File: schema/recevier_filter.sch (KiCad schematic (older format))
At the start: 14 parts, among them U7 LM358, U8 LM393

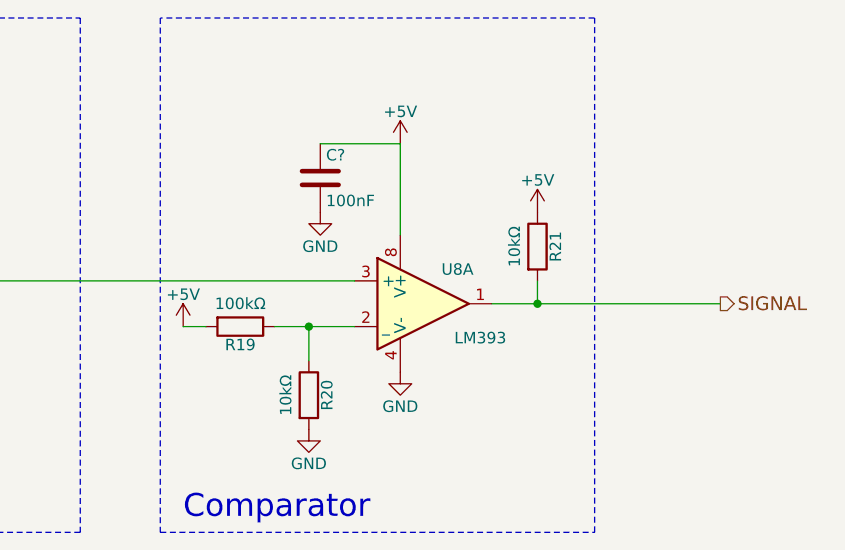
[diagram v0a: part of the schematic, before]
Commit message: Reception: schmidt trigger
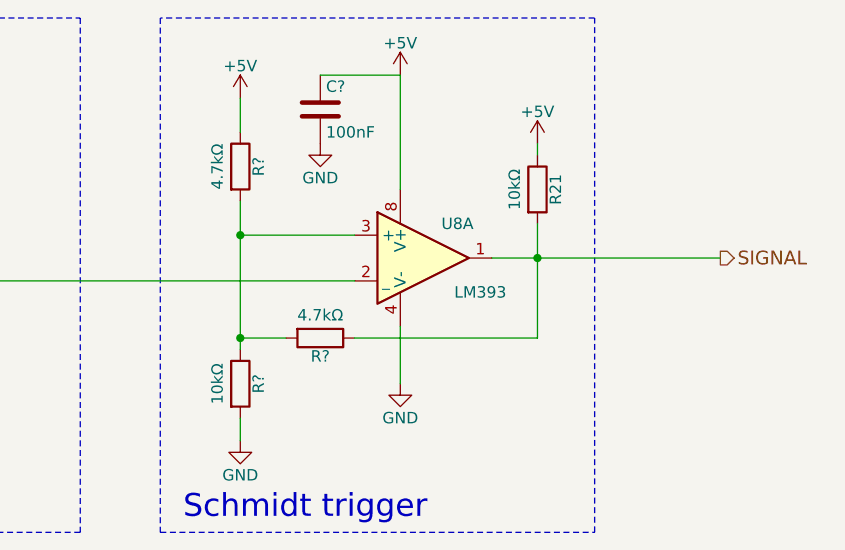
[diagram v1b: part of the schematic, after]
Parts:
- removed R19: 100kΩ, symbol R
- removed R20: 10kΩ, symbol R
- added R? (x2): 4.7kΩ, symbol R
- added R?: 10kΩ, symbol R
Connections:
- net +5V: now also R?.1
- net GND: now also R?.2
- net SIGNAL: now also R?.1
- net at R18.1, U?.1: now also U8.2 (_); no longer U8.3 (+)
- new net: R?.1, R?.2, R?.2, U8.3 (+)
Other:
- note added: "Schmidt trigger"
- note removed: "Comparator"
- moved on the sheet: C?, R21, U8A
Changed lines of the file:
@@
 Comment4 ""
 $EndDescr
-Text HLabel 9700 3650 2    60   Output ~ 0
+Text HLabel 9700 3450 2    60   Output ~ 0
 SIGNAL
 $Comp
@@
 L LM393 U8
 U 1 1 5924C9D9
-P 8400 3650
-F 0 "U8" H 8550 3800 50  0000 C CNN
-F 1 "LM393" H 8650 3500 50  0000 C CNN
-F 2 "" H 8400 3650 50  0000 C CNN
-F 3 "" H 8400 3650 50  0000 C CNN
-	1    8400 3650
-	1    0    0    -1
-$EndComp
-$Comp
-L R R19
-U 1 1 5924CC18
-P 7600 3750
-F 0 "R19" V 7680 3750 50  0000 C CNN
-F 1 "100kΩ" V 7500 3750 50  0000 C CNN
-F 2 "" V 7530 3750 50  0000 C CNN
-F 3 "" H 7600 3750 50  0000 C CNN
-	1    7600 3750
-	0    1    1    0
-$EndComp
-$Comp
-L R R20
-U 1 1 5924CC6A
-P 7900 4050
-F 0 "R20" V 7980 4050 50  0000 C CNN
-F 1 "10kΩ" V 7800 4050 50  0000 C CNN
-F 2 "" V 7830 4050 50  0000 C CNN
-F 3 "" H 7900 4050 50  0000 C CNN
-	1    7900 4050
+P 8400 3450
+F 0 "U8" H 8550 3600 50  0000 C CNN
+F 1 "LM393" H 8650 3300 50  0000 C CNN
+F 2 "" H 8400 3450 50  0000 C CNN
+F 3 "" H 8400 3450 50  0000 C CNN
+	1    8400 3450
 	1    0    0    -1
 $EndComp
@@
 L GND #PWR23
 U 1 1 5924CCA3
-P 7900 4200
-F 0 "#PWR23" H 7900 3950 50  0001 C CNN
-F 1 "GND" H 7900 4050 50  0000 C CNN
-F 2 "" H 7900 4200 50  0000 C CNN
-F 3 "" H 7900 4200 50  0000 C CNN
-	1    7900 4200
+P 7600 4250
+F 0 "#PWR23" H 7600 4000 50  0001 C CNN
+F 1 "GND" H 7600 4100 50  0000 C CNN
+F 2 "" H 7600 4250 50  0000 C CNN
+F 3 "" H 7600 4250 50  0000 C CNN
+	1    7600 4250
 	1    0    0    -1
 $EndComp
@@
 L GND #PWR25
 U 1 1 5924CE19
-P 8300 3950
-F 0 "#PWR25" H 8300 3700 50  0001 C CNN
-F 1 "GND" H 8300 3800 50  0000 C CNN
-F 2 "" H 8300 3950 50  0000 C CNN
-F 3 "" H 8300 3950 50  0000 C CNN
-	1    8300 3950
+P 8300 4000
+F 0 "#PWR25" H 8300 3750 50  0001 C CNN
+F 1 "GND" H 8300 3850 50  0000 C CNN
+F 2 "" H 8300 4000 50  0000 C CNN
+F 3 "" H 8300 4000 50  0000 C CNN
+	1    8300 4000
 	1    0    0    -1
 $EndComp
@@
 L +5V #PWR24
 U 1 1 5924CE97
-P 8300 2950
-F 0 "#PWR24" H 8300 2800 50  0001 C CNN
-F 1 "+5V" H 8300 3090 50  0000 C CNN
-F 2 "" H 8300 2950 50  0000 C CNN
-F 3 "" H 8300 2950 50  0000 C CNN
-	1    8300 2950
+P 8300 2650
+F 0 "#PWR24" H 8300 2500 50  0001 C CNN
+F 1 "+5V" H 8300 2790 50  0000 C CNN
+F 2 "" H 8300 2650 50  0000 C CNN
+F 3 "" H 8300 2650 50  0000 C CNN
+	1    8300 2650
 	1    0    0    -1
 $EndComp
@@
 L +5V #PWR22
 U 1 1 5924CFDF
-P 7350 3750
-F 0 "#PWR22" H 7350 3600 50  0001 C CNN
-F 1 "+5V" H 7350 3890 50  0000 C CNN
-F 2 "" H 7350 3750 50  0000 C CNN
-F 3 "" H 7350 3750 50  0000 C CNN
-	1    7350 3750
-	1    0    0    -1
-$EndComp
-Wire Wire Line
-	7350 3750 7450 3750
-Wire Wire Line
-	7750 3750 8100 3750
-Wire Wire Line
-	7900 3900 7900 3750
-Connection ~ 7900 3750
-Wire Wire Line
-	8700 3650 9700 3650
+P 7600 2750
+F 0 "#PWR22" H 7600 2600 50  0001 C CNN
+F 1 "+5V" H 7600 2890 50  0000 C CNN
+F 2 "" H 7600 2750 50  0000 C CNN
+F 3 "" H 7600 2750 50  0000 C CNN
+	1    7600 2750
+	1    0    0    -1
+$EndComp
 Wire Notes Line
 	7250 2400 7250 4650
@@
 	9150 2400 7250 2400
 Text Notes 7350 4600 0    100  ~ 0
-Comparator
+Schmidt trigger
 $Comp
 L R R21
 U 1 1 5924DDAD
-P 8900 3400
-F 0 "R21" V 8980 3400 50  0000 C CNN
-F 1 "10kΩ" V 8800 3400 50  0000 C CNN
-F 2 "" V 8830 3400 50  0000 C CNN
-F 3 "" H 8900 3400 50  0000 C CNN
-	1    8900 3400
-	1    0    0    -1
-$EndComp
-Wire Wire Line
-	8900 3550 8900 3650
-Connection ~ 8900 3650
+P 8900 3150
+F 0 "R21" V 8980 3150 50  0000 C CNN
+F 1 "10kΩ" V 8800 3150 50  0000 C CNN
+F 2 "" V 8830 3150 50  0000 C CNN
+F 3 "" H 8900 3150 50  0000 C CNN
+	1    8900 3150
+	1    0    0    -1
+$EndComp
 $Comp
 L +5V #PWR26
 U 1 1 5924DE3C
-P 8900 3250
-F 0 "#PWR26" H 8900 3100 50  0001 C CNN
-F 1 "+5V" H 8900 3390 50  0000 C CNN
-F 2 "" H 8900 3250 50  0000 C CNN
-F 3 "" H 8900 3250 50  0000 C CNN
-	1    8900 3250
+P 8900 2950
+F 0 "#PWR26" H 8900 2800 50  0001 C CNN
+F 1 "+5V" H 8900 3090 50  0000 C CNN
+F 2 "" H 8900 2950 50  0000 C CNN
+F 3 "" H 8900 2950 50  0000 C CNN
+	1    8900 2950
 	1    0    0    -1
 $EndComp
@@
 L C C?
 U 1 1 59253FAB
-P 7950 3100
-F 0 "C?" H 7975 3200 50  0000 L CNN
-F 1 "100nF" H 7975 3000 50  0000 L CNN
-F 2 "" H 7988 2950 50  0000 C CNN
-F 3 "" H 7950 3100 50  0000 C CNN
-	1    7950 3100
+P 7950 2800
+F 0 "C?" H 7975 2900 50  0000 L CNN
+F 1 "100nF" H 7975 2700 50  0000 L CNN
+F 2 "" H 7988 2650 50  0000 C CNN
+F 3 "" H 7950 2800 50  0000 C CNN
+	1    7950 2800
 	1    0    0    -1
 $EndComp
@@
 L GND #PWR?
 U 1 1 5925407F
-P 7950 3250
-F 0 "#PWR?" H 7950 3000 50  0001 C CNN
-F 1 "GND" H 7950 3100 50  0000 C CNN
-F 2 "" H 7950 3250 50  0000 C CNN
-F 3 "" H 7950 3250 50  0000 C CNN
-	1    7950 3250
-	1    0    0    -1
-$EndComp
-Wire Wire Line
-	7950 2950 8300 2950
-Wire Wire Line
-	8300 2950 8300 3350
+P 7950 2950
+F 0 "#PWR?" H 7950 2700 50  0001 C CNN
+F 1 "GND" H 7950 2800 50  0000 C CNN
+F 2 "" H 7950 2950 50  0000 C CNN
+F 3 "" H 7950 2950 50  0000 C CNN
+	1    7950 2950
+	1    0    0    -1
+$EndComp
+Wire Wire Line
+	7950 2650 8300 2650
+$Comp
+L R R?
+U 1 1 592F2986
+P 7600 3050
+F 0 "R?" V 7680 3050 50  0000 C CNN
+F 1 "4.7kΩ" V 7500 3050 50  0000 C CNN
+F 2 "" V 7530 3050 50  0000 C CNN
+F 3 "" H 7600 3050 50  0000 C CNN
+	1    7600 3050
+	1    0    0    -1
+$EndComp
+$Comp
+L R R?
+U 1 1 592F2B41
+P 7600 4000
+F 0 "R?" V 7680 4000 50  0000 C CNN
+F 1 "10kΩ" V 7500 4000 50  0000 C CNN
+F 2 "" V 7530 4000 50  0000 C CNN
+F 3 "" H 7600 4000 50  0000 C CNN
+	1    7600 4000
+	1    0    0    -1
+$EndComp
+Wire Wire Line
+	8700 3450 9700 3450
+Wire Wire Line
+	8900 3300 8900 3800
+Connection ~ 8900 3450
+Wire Wire Line
+	7600 2750 7600 2900
+Wire Wire Line
+	7600 3200 7600 3850
+Wire Wire Line
+	7600 3350 8100 3350
+Connection ~ 7600 3350
+Wire Wire Line
+	7600 4150 7600 4250
+Connection ~ 7600 3800
+Wire Wire Line
+	8300 3750 8300 4000
+$Comp
+L R R?
+U 1 1 592F300B
+P 7950 3800
+F 0 "R?" V 8030 3800 50  0000 C CNN
+F 1 "4.7kΩ" V 7850 3800 50  0000 C CNN
+F 2 "" V 7880 3800 50  0000 C CNN
+F 3 "" H 7950 3800 50  0000 C CNN
+	1    7950 3800
+	0    1    1    0
+$EndComp
+Wire Wire Line
+	7600 3800 7800 3800
+Wire Wire Line
+	8900 3800 8100 3800
+Wire Wire Line
+	8900 2950 8900 3000
+Wire Wire Line
+	8300 2650 8300 3150
 $EndSCHEMATC
